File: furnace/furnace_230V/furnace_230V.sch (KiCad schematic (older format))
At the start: 10 parts, among them J1 , J2 , J3 IDC-6

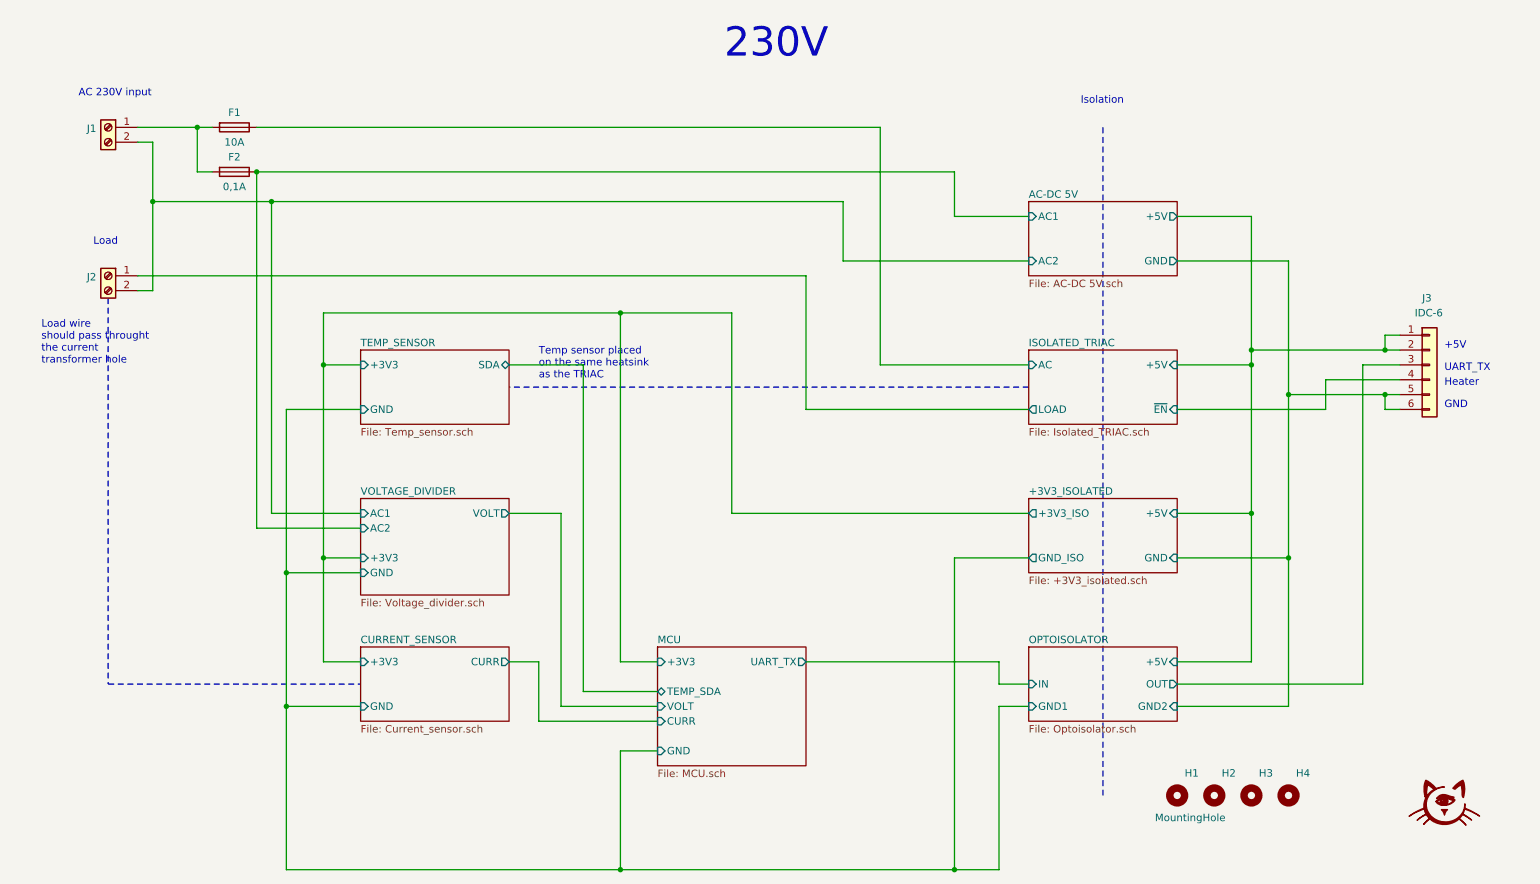
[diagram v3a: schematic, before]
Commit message: Add files via upload
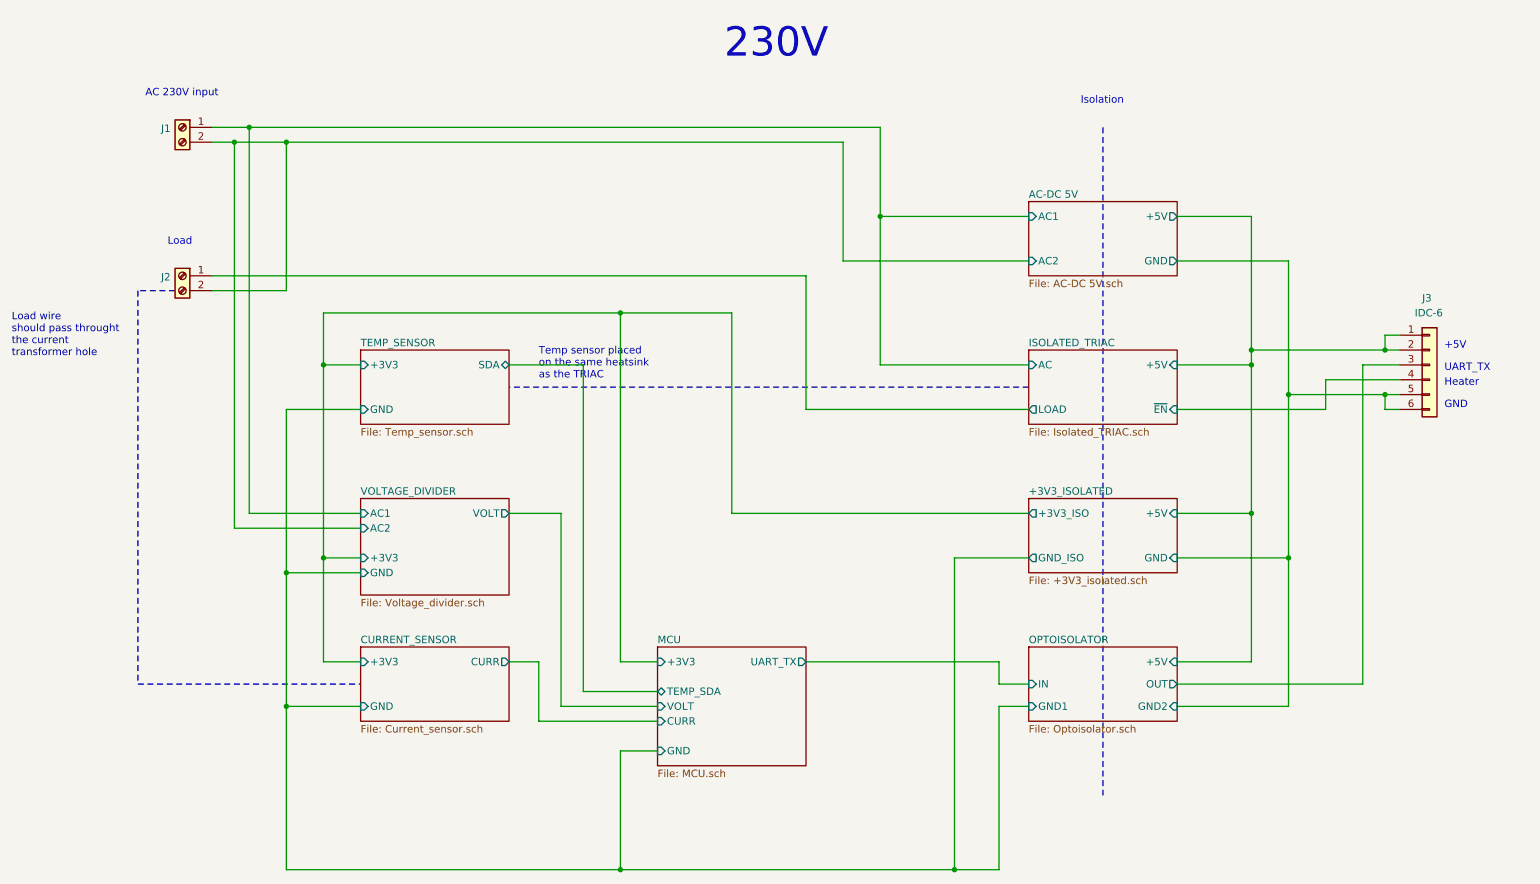
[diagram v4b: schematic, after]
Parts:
- removed F1: 10A, Fuse:Fuseholder_Cylinder-5x20mm_Stelvio-Kontek_PTF78_Horizontal_Open, symbol furnace_230V-rescue:Fuse-Device
- removed F2: 0,1A, Fuse:Fuseholder_Cylinder-5x20mm_Stelvio-Kontek_PTF78_Horizontal_Open, symbol furnace_230V-rescue:Fuse-Device
- removed G1: LOGO, furnace_230V:stamp, symbol stamp:LOGO
- removed H1, H2, H3, H4: MountingHole, furnace_230V:hole_D3.5mm, symbol Mechanical:MountingHole
- J1, J2: footprint furnace_230V:KF7.62-2P -> (none)
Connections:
- net AC-DC 5V/AC1: now also J1.1 (Pin_1)
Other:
- moved on the sheet: J1, J2
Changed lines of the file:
@@
 L furnace_230V-rescue:Screw_Terminal_01x02-Connector J1
 U 1 1 60AAEFEC
-P 1300 1500
-F 0 "J1" H 1380 1492 50  0000 L CNN
-F 1 " " H 1380 1401 50  0000 L CNN
-F 2 "furnace_230V:KF7.62-2P" H 1300 1500 50  0001 C CNN
-F 3 "~" H 1300 1500 50  0001 C CNN
-	1    1300 1500
+P 1800 1500
+F 0 "J1" H 1880 1492 50  0000 L CNN
+F 1 " " H 1880 1401 50  0000 L CNN
+F 2 "" H 1800 1500 50  0001 C CNN
+F 3 "~" H 1800 1500 50  0001 C CNN
+	1    1800 1500
 	-1   0    0    -1
 $EndComp
@@
 L furnace_230V-rescue:Screw_Terminal_01x02-Connector J2
 U 1 1 60AB629C
-P 1300 2500
-F 0 "J2" H 1380 2492 50  0000 L CNN
-F 1 " " H 1380 2401 50  0000 L CNN
-F 2 "furnace_230V:KF7.62-2P" H 1300 2500 50  0001 C CNN
-F 3 "~" H 1300 2500 50  0001 C CNN
-	1    1300 2500
+P 1800 2500
+F 0 "J2" H 1880 2492 50  0000 L CNN
+F 1 " " H 1880 2401 50  0000 L CNN
+F 2 "" H 1800 2500 50  0001 C CNN
+F 3 "~" H 1800 2500 50  0001 C CNN
+	1    1800 2500
 	-1   0    0    -1
 $EndComp
@@
 F4 "GND" I L 3000 5400 50
 $EndSheet
-Text Notes 1100 1300 0    50   ~ 0
+Text Notes 1550 1300 0    50   ~ 0
 AC 230V input
 Wire Notes Line rgb(255, 0, 0)
 	8000 1500 8000 6000
 Wire Notes Line
-	1300 2650 1300 5250
+	1750 2600 1500 2600
 Wire Notes Line
-	1300 5250 3000 5250
+	1500 2600 1500 5250
+Wire Notes Line
+	1500 5250 3000 5250
 Wire Notes Line
 	7500 3250 4000 3250
 Text Notes 7850 1350 0    50   ~ 0
 Isolation
-Text Notes 850  3100 0    50   ~ 0
+Text Notes 650  3050 0    50   ~ 0
 Load wire \nshould pass throught\nthe current \ntransformer hole
 Text Notes 4200 3200 0    50   ~ 0
 Temp sensor placed \non the same heatsink\nas the TRIAC
-Text Notes 1200 2300 0    50   ~ 0
+Text Notes 1700 2300 0    50   ~ 0
 Load
 Wire Wire Line
+	6500 1500 6500 2100
+Wire Wire Line
+	6500 2100 7500 2100
+Wire Wire Line
 	7500 3100 6500 3100
 Wire Wire Line
+	6500 3100 6500 2100
+Connection ~ 6500 2100
+Wire Wire Line
 	7500 3400 6000 3400
 Wire Wire Line
 	7500 2400 6250 2400
 Wire Wire Line
-	6250 2400 6250 2000
+	6250 2400 6250 1600
+Wire Wire Line
+	2000 1500 2250 1500
+Wire Wire Line
+	2000 1600 2150 1600
 Wire Wire Line
 	6000 3400 6000 2500
+Wire Wire Line
+	6000 2500 2000 2500
+Wire Wire Line
+	2000 2600 2500 2600
+Wire Wire Line
+	2500 2600 2500 1600
+Connection ~ 2500 1600
+Wire Wire Line
+	2500 1600 6250 1600
 Text Notes 6150 1050 2    197  ~ 0
 230V
@@
 	2500 5400 2500 4500
 Wire Wire Line
-	3000 4100 2400 4100
-Wire Wire Line
-	2400 4100 2400 2000
-Wire Wire Line
-	3000 4200 2300 4200
-Wire Wire Line
-	2300 4200 2300 1800
+	3000 4100 2250 4100
+Wire Wire Line
+	2250 4100 2250 1500
+Connection ~ 2250 1500
+Wire Wire Line
+	2250 1500 6500 1500
+Wire Wire Line
+	3000 4200 2150 4200
+Wire Wire Line
+	2150 4200 2150 1600
+Connection ~ 2150 1600
+Wire Wire Line
+	2150 1600 2500 1600
 Wire Wire Line
 	5000 5700 4750 5700
@@
 Wire Wire Line
 	9900 3300 9250 3300
-$Comp
-L stamp:LOGO G1
-U 1 1 610EDF1B
-P 10300 6050
-F 0 "G1" H 10300 5928 60  0001 C CNN
-F 1 "LOGO" H 10300 6172 60  0001 C CNN
-F 2 "furnace_230V:stamp" H 10300 6050 50  0001 C CNN
-F 3 "" H 10300 6050 50  0001 C CNN
-	1    10300 6050
-	1    0    0    -1
-$EndComp
-$Comp
-L Mechanical:MountingHole H1
-U 1 1 6110929D
-P 8500 6000
-F 0 "H1" H 8550 6150 50  0000 L CNN
-F 1 "MountingHole" H 8350 5850 50  0000 L CNN
-F 2 "furnace_230V:hole_D3.5mm" H 8500 6000 50  0001 C CNN
-F 3 "~" H 8500 6000 50  0001 C CNN
-	1    8500 6000
-	1    0    0    -1
-$EndComp
-$Comp
-L Mechanical:MountingHole H2
-U 1 1 6110B2E7
-P 8750 6000
-F 0 "H2" H 8800 6150 50  0000 L CNN
-F 1 "MountingHole" H 8600 5850 50  0001 L CNN
-F 2 "furnace_230V:hole_D3.5mm" H 8750 6000 50  0001 C CNN
-F 3 "~" H 8750 6000 50  0001 C CNN
-	1    8750 6000
-	1    0    0    -1
-$EndComp
-$Comp
-L Mechanical:MountingHole H3
-U 1 1 6110B4DC
-P 9000 6000
-F 0 "H3" H 9050 6150 50  0000 L CNN
-F 1 "MountingHole" H 8850 5850 50  0001 L CNN
-F 2 "furnace_230V:hole_D3.5mm" H 9000 6000 50  0001 C CNN
-F 3 "~" H 9000 6000 50  0001 C CNN
-	1    9000 6000
-	1    0    0    -1
-$EndComp
-$Comp
-L Mechanical:MountingHole H4
-U 1 1 6110B613
-P 9250 6000
-F 0 "H4" H 9300 6150 50  0000 L CNN
-F 1 "MountingHole" H 9100 5850 50  0001 L CNN
-F 2 "furnace_230V:hole_D3.5mm" H 9250 6000 50  0001 C CNN
-F 3 "~" H 9250 6000 50  0001 C CNN
-	1    9250 6000
-	1    0    0    -1
-$EndComp
-$Comp
-L furnace_230V-rescue:Fuse-Device F?
-U 1 1 61103E7E
-P 2150 1800
-AR Path="/60AABABA/61103E7E" Ref="F?"  Part="1"
-AR Path="/61103E7E" Ref="F2"  Part="1"
-F 0 "F2" V 2050 1800 50  0000 C CNN
-F 1 "0,1A" V 2250 1800 50  0000 C CNN
-F 2 "Fuse:Fuseholder_Cylinder-5x20mm_Stelvio-Kontek_PTF78_Horizontal_Open" V 2080 1800 50  0001 C CNN
-F 3 "~" H 2150 1800 50  0001 C CNN
-	1    2150 1800
-	0    1    1    0
-$EndComp
-$Comp
-L furnace_230V-rescue:Fuse-Device F?
-U 1 1 61107140
-P 2150 1500
-AR Path="/60AAE0B8/61107140" Ref="F?"  Part="1"
-AR Path="/61107140" Ref="F1"  Part="1"
-F 0 "F1" V 2050 1500 50  0000 C CNN
-F 1 "10A" V 2250 1500 50  0000 C CNN
-F 2 "Fuse:Fuseholder_Cylinder-5x20mm_Stelvio-Kontek_PTF78_Horizontal_Open" V 2080 1500 50  0001 C CNN
-F 3 "~" H 2150 1500 50  0001 C CNN
-	1    2150 1500
-	0    1    1    0
-$EndComp
-Wire Wire Line
-	6500 1500 6500 3100
-Wire Wire Line
-	1600 2600 1600 2000
-Wire Wire Line
-	1600 1600 1500 1600
-Wire Wire Line
-	6250 2000 2400 2000
-Connection ~ 1600 2000
-Wire Wire Line
-	1600 2000 1600 1600
-Connection ~ 2400 2000
-Wire Wire Line
-	2400 2000 1600 2000
-Wire Wire Line
-	1500 1500 1900 1500
-Wire Wire Line
-	2000 1800 1900 1800
-Wire Wire Line
-	1900 1800 1900 1500
-Connection ~ 1900 1500
-Wire Wire Line
-	1900 1500 2000 1500
-Wire Wire Line
-	2300 1500 6500 1500
-Wire Wire Line
-	2300 1800 7000 1800
-Wire Wire Line
-	7000 1800 7000 2100
-Wire Wire Line
-	7000 2100 7500 2100
-Connection ~ 2300 1800
-Wire Wire Line
-	1600 2600 1500 2600
-Wire Wire Line
-	1500 2500 6000 2500
 $EndSCHEMATC
